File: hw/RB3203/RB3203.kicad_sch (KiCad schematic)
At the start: 6 parts

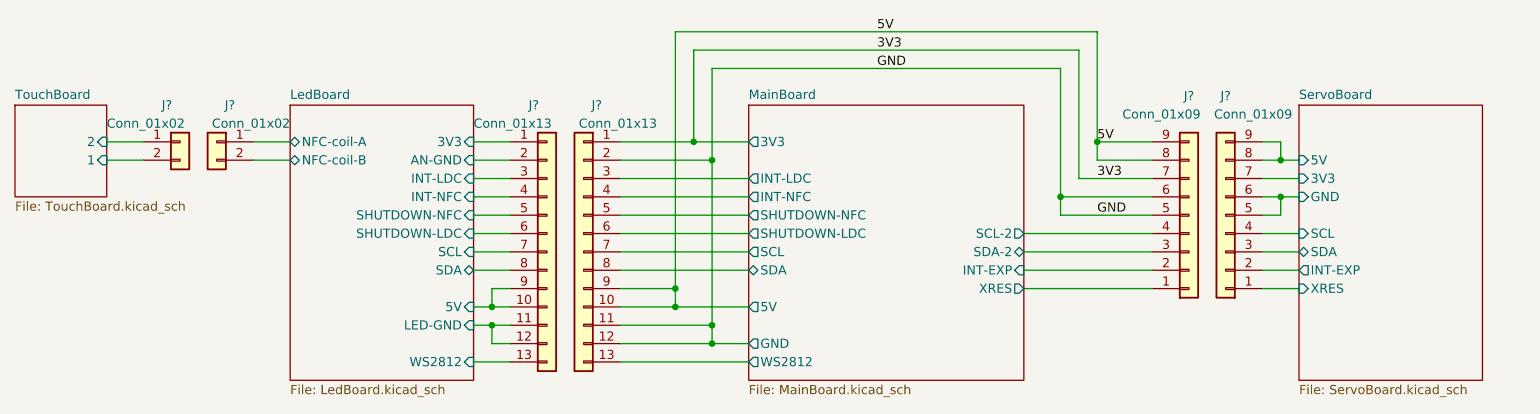
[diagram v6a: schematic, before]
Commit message: Wip
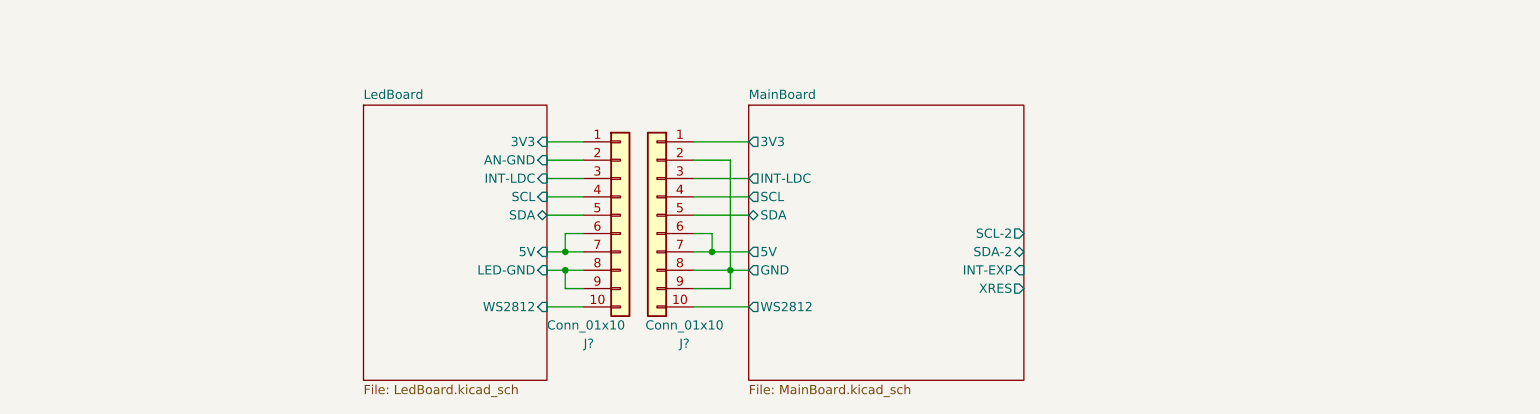
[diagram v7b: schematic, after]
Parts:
- removed J? (x2): Conn_01x13, symbol Connector_Generic:Conn_01x13
- removed J? (x2): Conn_01x09, symbol Connector_Generic:Conn_01x09
- removed J? (x2): Conn_01x02, symbol Connector_Generic:Conn_01x02
- added J? (x2): Conn_01x10, symbol Connector_Generic:Conn_01x10
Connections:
- net LedBoard/3V3: now also J?.1 (Pin_1)
- net LedBoard/5V: now also J?.6 (Pin_6), J?.7 (Pin_7)
- net LedBoard/AN-GND: now also J?.2 (Pin_2)
- net LedBoard/INT-LDC: now also J?.3 (Pin_3)
- net LedBoard/LED-GND: now also J?.8 (Pin_8), J?.9 (Pin_9)
- net LedBoard/SCL: now also J?.4 (Pin_4)
- net LedBoard/SDA: now also J?.5 (Pin_5)
- net LedBoard/WS2812: now also J?.10 (Pin_10)
- net MainBoard/INT-LDC: now also J?.3 (Pin_3)
- net MainBoard/SCL: now also J?.4 (Pin_4)
- net MainBoard/SDA: now also J?.5 (Pin_5)
- net MainBoard/WS2812: now also J?.10 (Pin_10)
- new net MainBoard/3V3: J?.1 (Pin_1)
- new net MainBoard/5V: J?.6 (Pin_6), J?.7 (Pin_7)
- new net MainBoard/GND: J?.2 (Pin_2), J?.8 (Pin_8), J?.9 (Pin_9)
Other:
- removed sheet ServoBoard
- removed sheet TouchBoard
- sheet LedBoard ports: added none; removed INT-NFC, NFC-coil-A, NFC-coil-B, SHUTDOWN-LDC, SHUTDOWN-NFC
- sheet MainBoard ports: added none; removed INT-NFC, SHUTDOWN-LDC, SHUTDOWN-NFC
